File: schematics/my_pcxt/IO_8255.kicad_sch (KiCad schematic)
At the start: 2 parts, among them J4 Conn_02x40_Top_Bottom, U11 82C55A

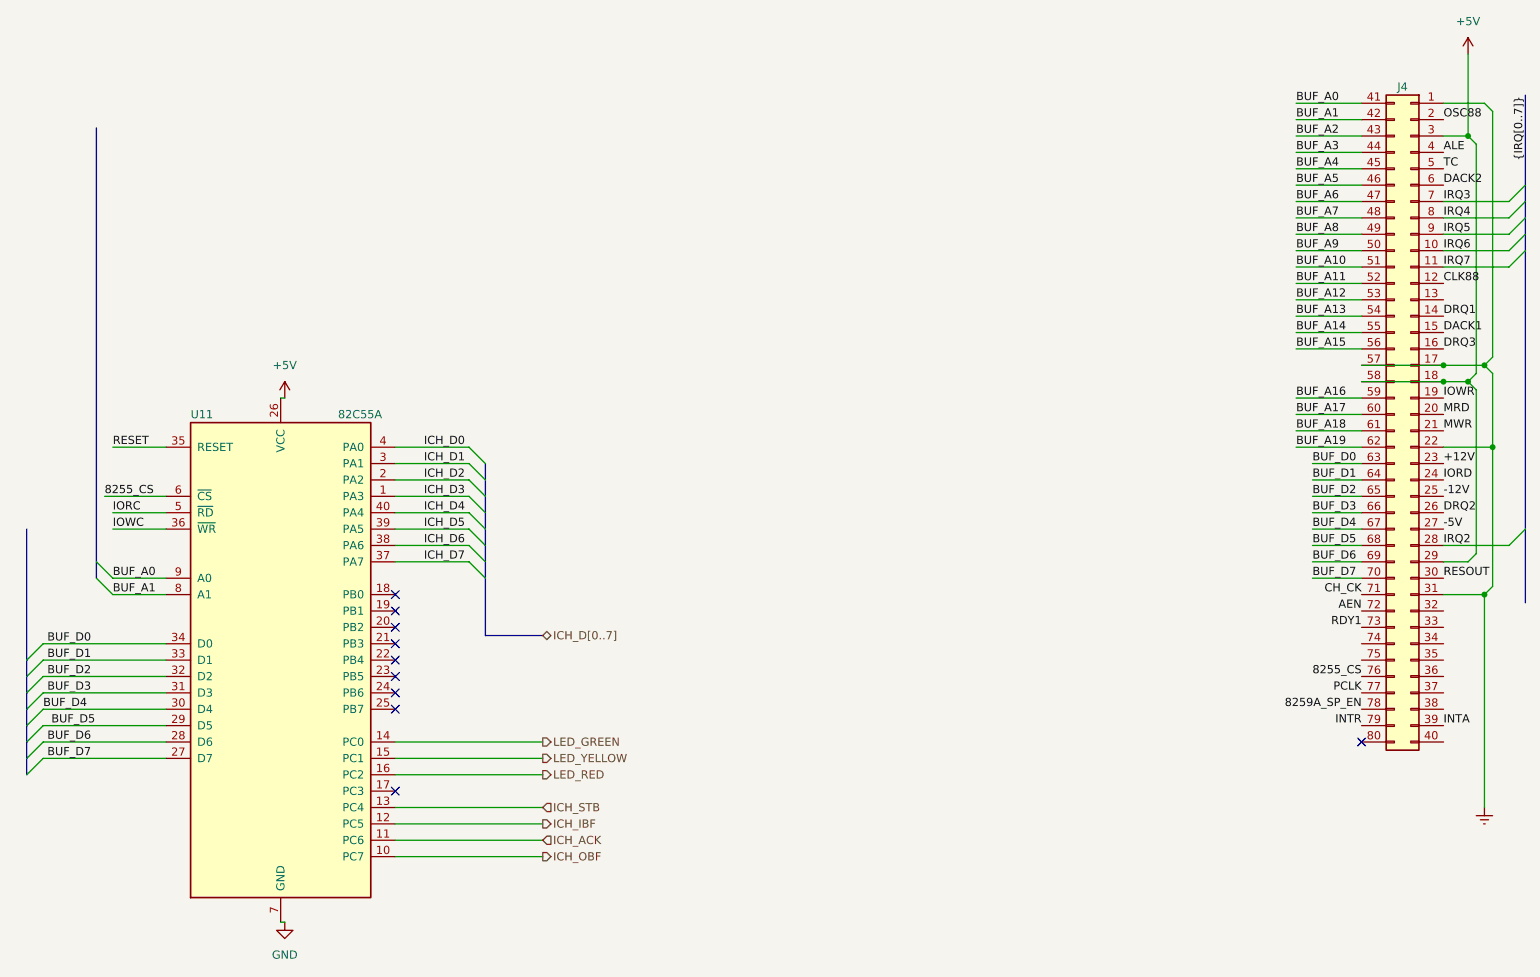
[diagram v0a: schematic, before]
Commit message: Updating code...
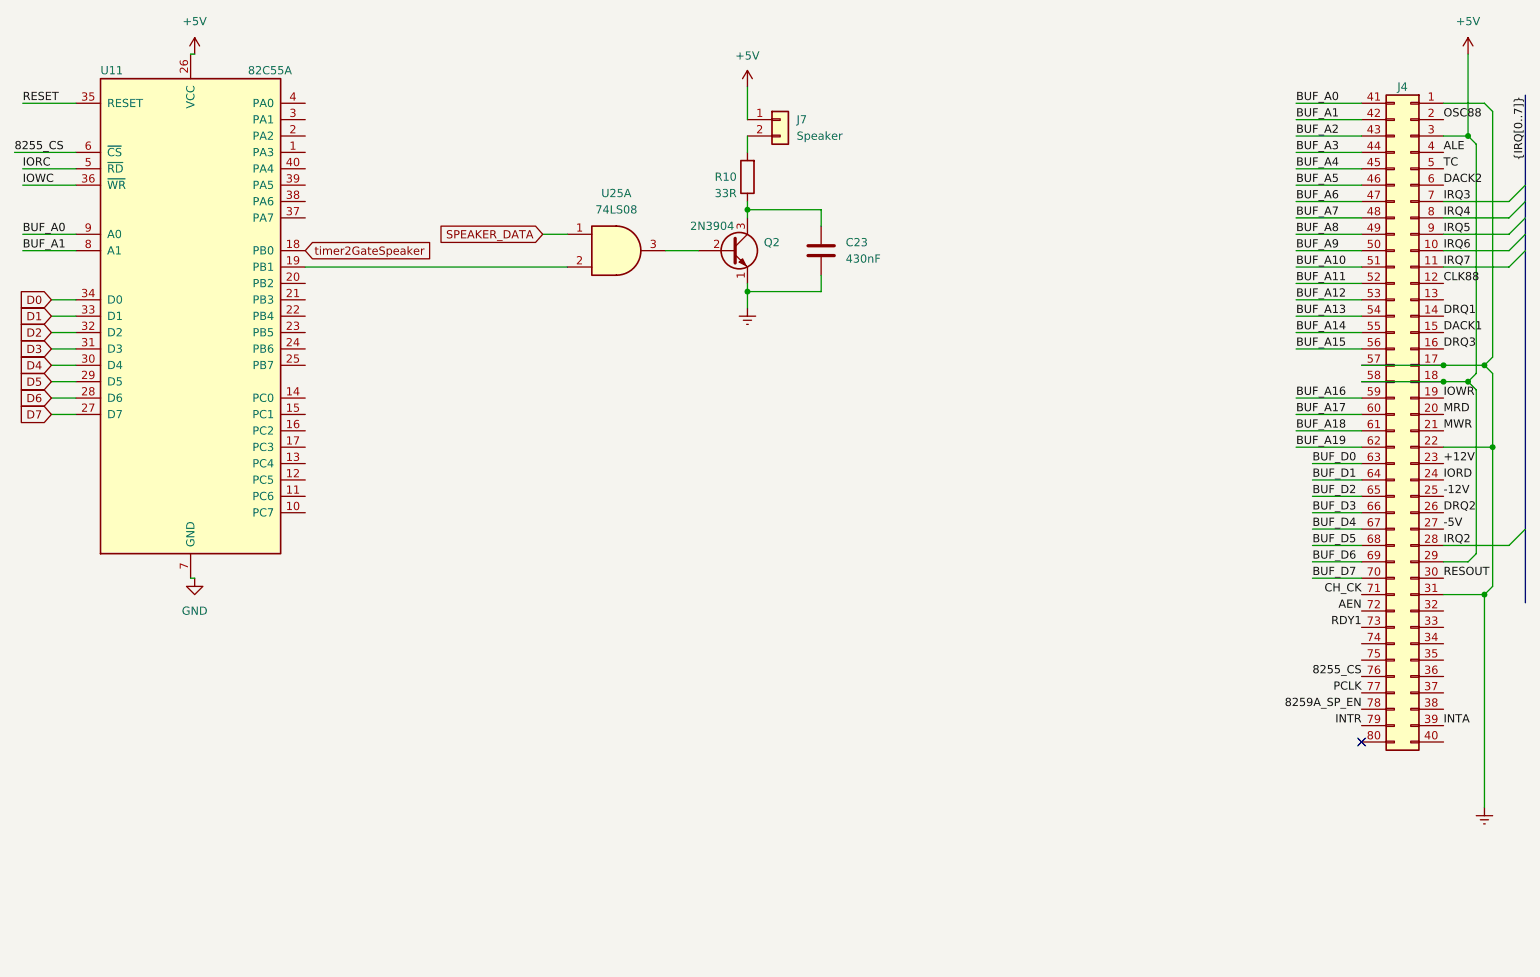
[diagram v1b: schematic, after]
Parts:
- added C23: 430nF, symbol Device:C
- added J7: Speaker, symbol Connector_Generic:Conn_01x02
- added Q2: 2N3904, Package_TO_SOT_THT:TO-92_Inline, symbol Transistor_BJT:2N3904
- added R10: 33R, symbol Device:R
- added U25: 74LS08, symbol 74xx:74LS08
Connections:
- net +5V: now also J7.1 (Pin_1)
- net BUF_D0: no longer U11.34 (D0)
- net BUF_D1: no longer U11.33 (D1)
- net BUF_D2: no longer U11.32 (D2)
- net BUF_D3: no longer U11.31 (D3)
- net BUF_D4: no longer U11.30 (D4)
- net BUF_D5: no longer U11.29 (D5)
- net BUF_D6: no longer U11.28 (D6)
- net BUF_D7: no longer U11.27 (D7)
- net GNDREF: now also C23.2, Q2.1 (E)
- net timer2GateSpeaker: now reaches U11.18 (PB0)
- net at U11.19 (PB1): now also U25.2
- net ICH_ACK: no longer names the net of U11.11 (PC6)
- net ICH_D0: no longer names the net of U11.4 (PA0)
- net ICH_D1: no longer names the net of U11.3 (PA1)
- net ICH_D2: no longer names the net of U11.2 (PA2)
- net ICH_D3: no longer names the net of U11.1 (PA3)
- net ICH_D4: no longer names the net of U11.40 (PA4)
- net ICH_D5: no longer names the net of U11.39 (PA5)
- net ICH_D6: no longer names the net of U11.38 (PA6)
- net ICH_D7: no longer names the net of U11.37 (PA7)
- net ICH_IBF: no longer names the net of U11.12 (PC5)
- net ICH_OBF: no longer names the net of U11.10 (PC7)
- net ICH_STB: no longer names the net of U11.13 (PC4)
- net LED_GREEN: no longer names the net of U11.14 (PC0)
- net LED_RED: no longer names the net of U11.16 (PC2)
- net LED_YELLOW: no longer names the net of U11.15 (PC1)
- new net: C23.1, Q2.3 (C), R10.1
- new net: Q2.2 (B), U25.3
- new net: J7.2 (Pin_2), R10.2
- new net D0: U11.34 (D0)
- new net D1: U11.33 (D1)
- new net D2: U11.32 (D2)
- new net D3: U11.31 (D3)
- new net D4: U11.30 (D4)
- new net D5: U11.29 (D5)
- new net D6: U11.28 (D6)
- new net D7: U11.27 (D7)
- new net SPEAKER_DATA: U25.1
- no-connect marks 10 -> 1
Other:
- moved on the sheet: U11
